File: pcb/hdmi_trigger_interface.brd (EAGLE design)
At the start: 78.7 x 63.5 mm, 58 parts, among them U1 TPD12S016PWR, U2 TPD12S016PWR, Y1 SI514

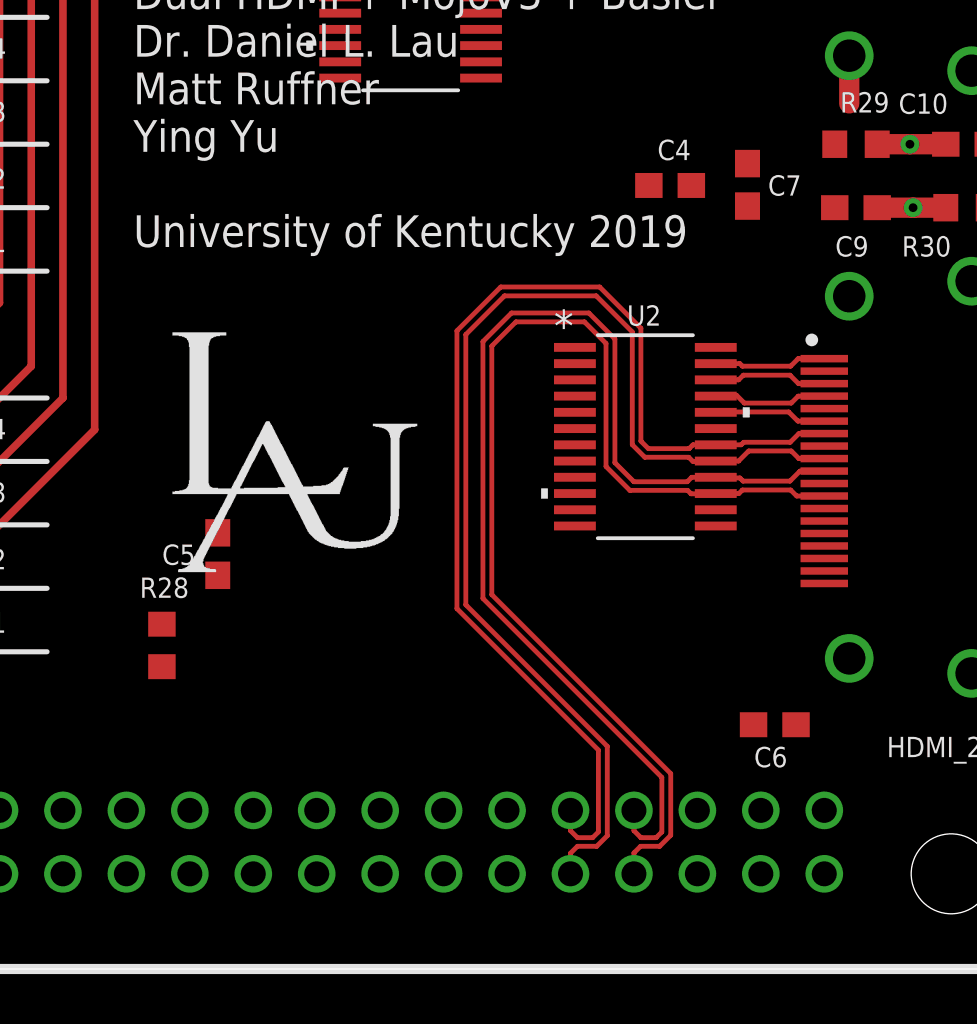
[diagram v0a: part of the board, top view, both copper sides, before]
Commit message: more routing
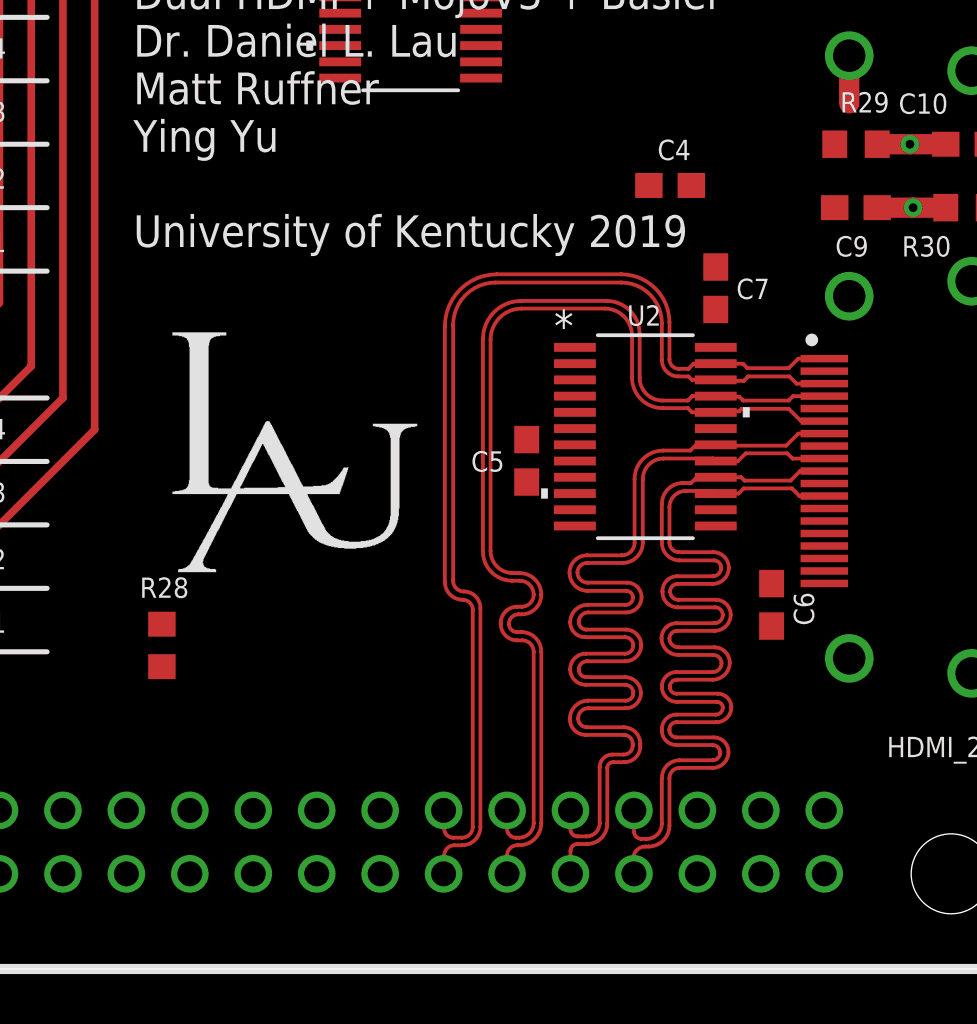
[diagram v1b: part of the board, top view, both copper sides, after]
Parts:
- moved C5 12.9 mm to (57.9, 20.3)
- moved C6 4.80 mm to (67.7, 14.6), turned to 270 degrees
- moved C7 4.33 mm to (65.5, 27.3)
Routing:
- net D22_P: track 4.51 -> 41.5 mm
- net D22_N: track 4.56 -> 41.5 mm
- net D12_N: track 4.50 -> 41.1 mm
- net D12_P: track 4.60 -> 41.1 mm
- net D02_N: track 45.7 -> 40.8 mm
- net D02_P: track 45.6 -> 40.8 mm
- net CLK2_P: track 44.9 -> 40.8 mm
- net CLK2_N: track 44.8 -> 40.7 mm
